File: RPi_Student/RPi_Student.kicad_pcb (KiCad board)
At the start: 2 copper layers, 65 x 56 mm, 11 parts, among them J1 Conn_01x02, J2 Conn_01x02, J3 Conn_01x03, J4 GPIO, J5 Conn_01x06, J6 Conn_01x04, J7 Conn_01x02_Male

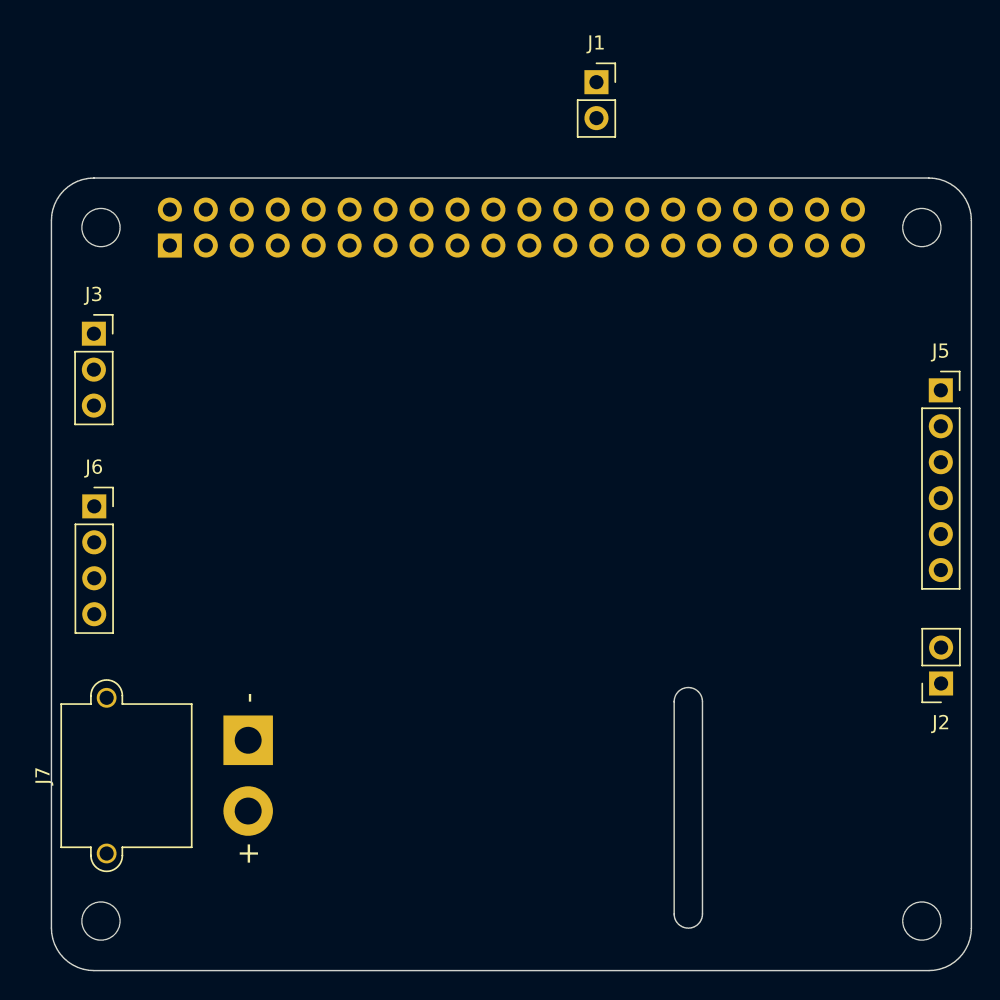
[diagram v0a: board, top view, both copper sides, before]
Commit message: Updated to account for new PCB design changes
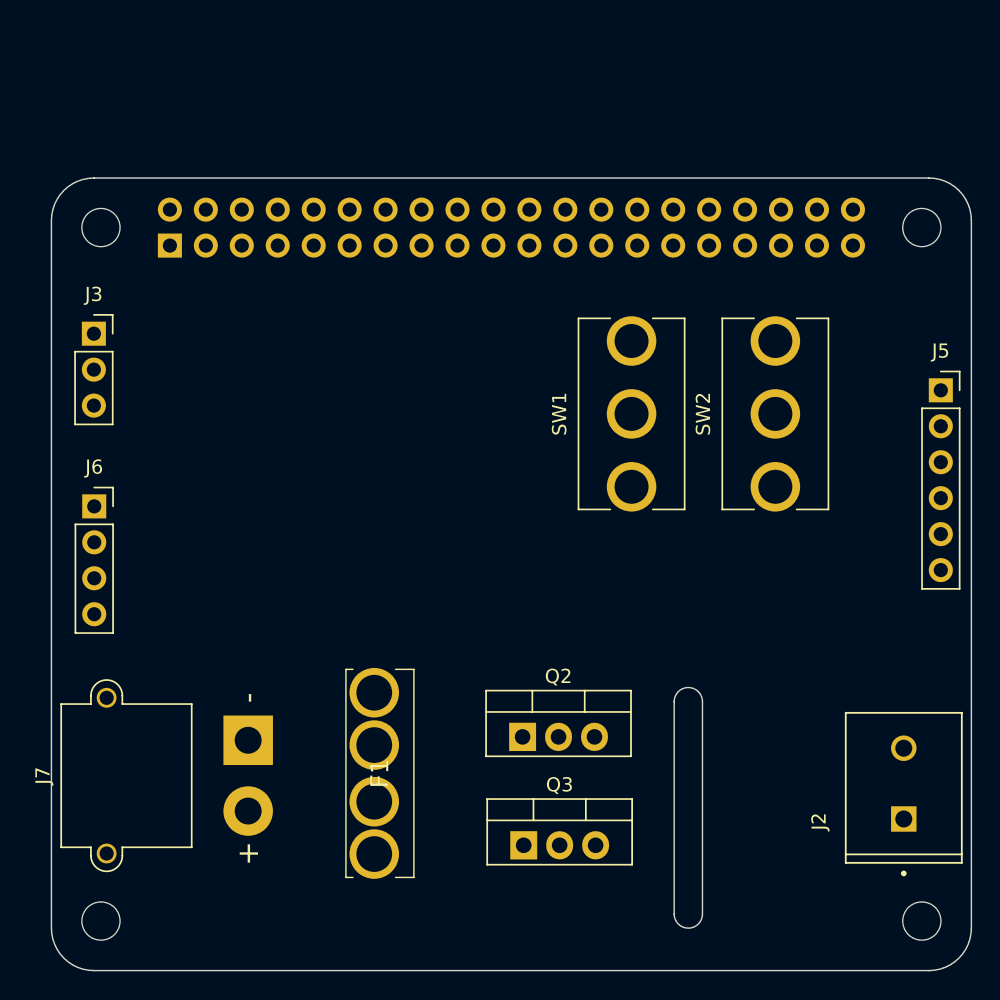
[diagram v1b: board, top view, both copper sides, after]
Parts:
- removed J1: Conn_01x02, Connector_PinSocket_2.54mm:PinSocket_1x02_P2.54mm_Vertical
- added F1: MCCQ-122, RPi_Hat:MCCQ122, F.Cu at (139.3, 122.5)
- added Q2: IRF9540N, Package_TO_SOT_THT:TO-220-3_Vertical, F.Cu at (149.8, 114.3)
- added Q3: IRF9540N, Package_TO_SOT_THT:TO-220-3_Vertical, F.Cu at (149.9, 121.9)
- added SW1: SW_SPDT, RPi_Hat:Switch_SPDT_Jaycar, F.Cu at (157.5, 91.4)
- added SW2: SW_SPDT, RPi_Hat:Switch_SPDT_Jaycar, F.Cu at (167.6, 91.4)
- J2: footprint Connector_PinSocket_2.54mm:PinSocket_1x02_P2.54mm_Vertical -> RPi_Hat:TE_282836-2
- moved J2 7.55 mm to (176.7, 117.6), turned to 90 degrees
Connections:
- J4 pad 4: /5v -> +5V
- J5 pad 4: +5V -> unconnected-(J5-Pad4)
- J7 pad 1: unconnected-(J7-Pad1) -> GND
- J7 pad 2: unconnected-(J7-Pad2) -> Net-(F1-Pad1)
